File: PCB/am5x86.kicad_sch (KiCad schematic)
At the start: 2 parts, among them U1 LFE5U-25F-6BG256C, U3 AM5x86 PQFP208

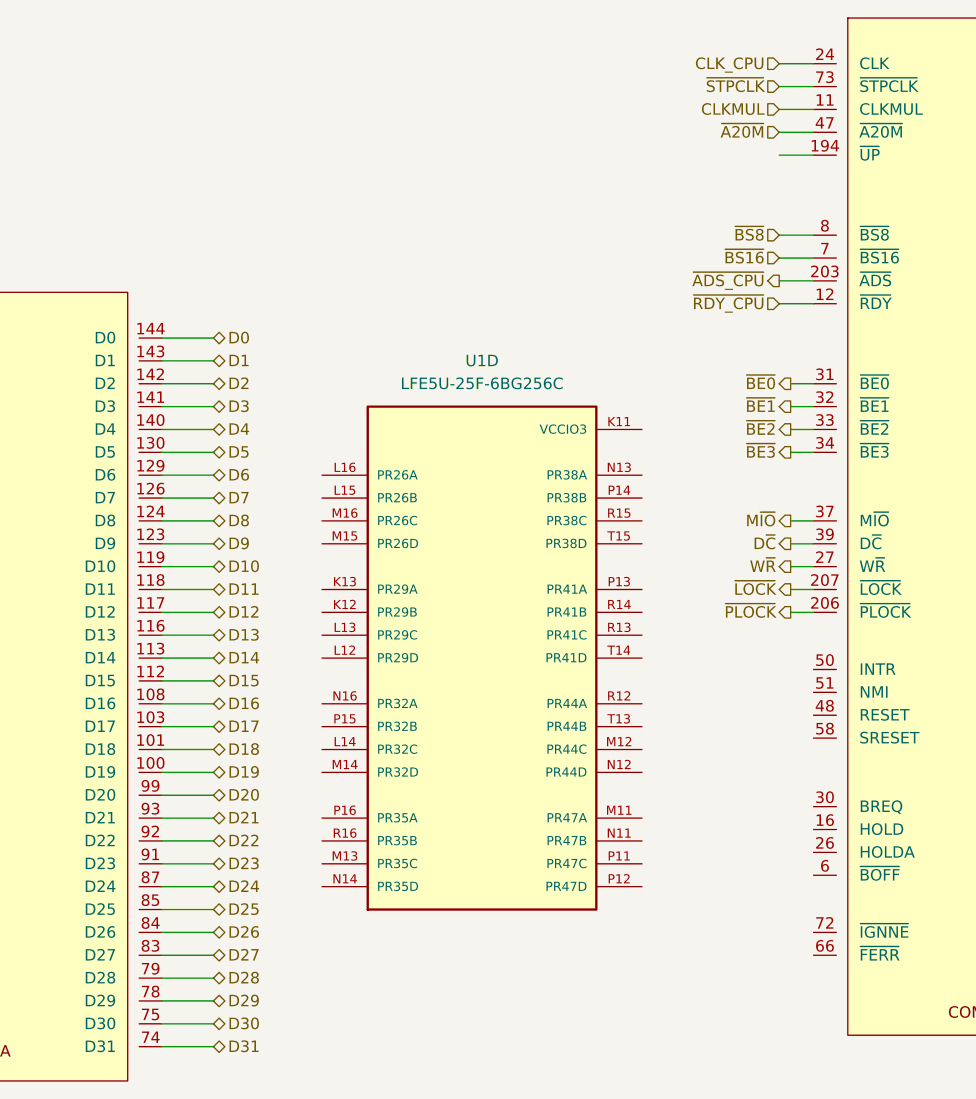
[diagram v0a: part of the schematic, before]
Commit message: More layout work
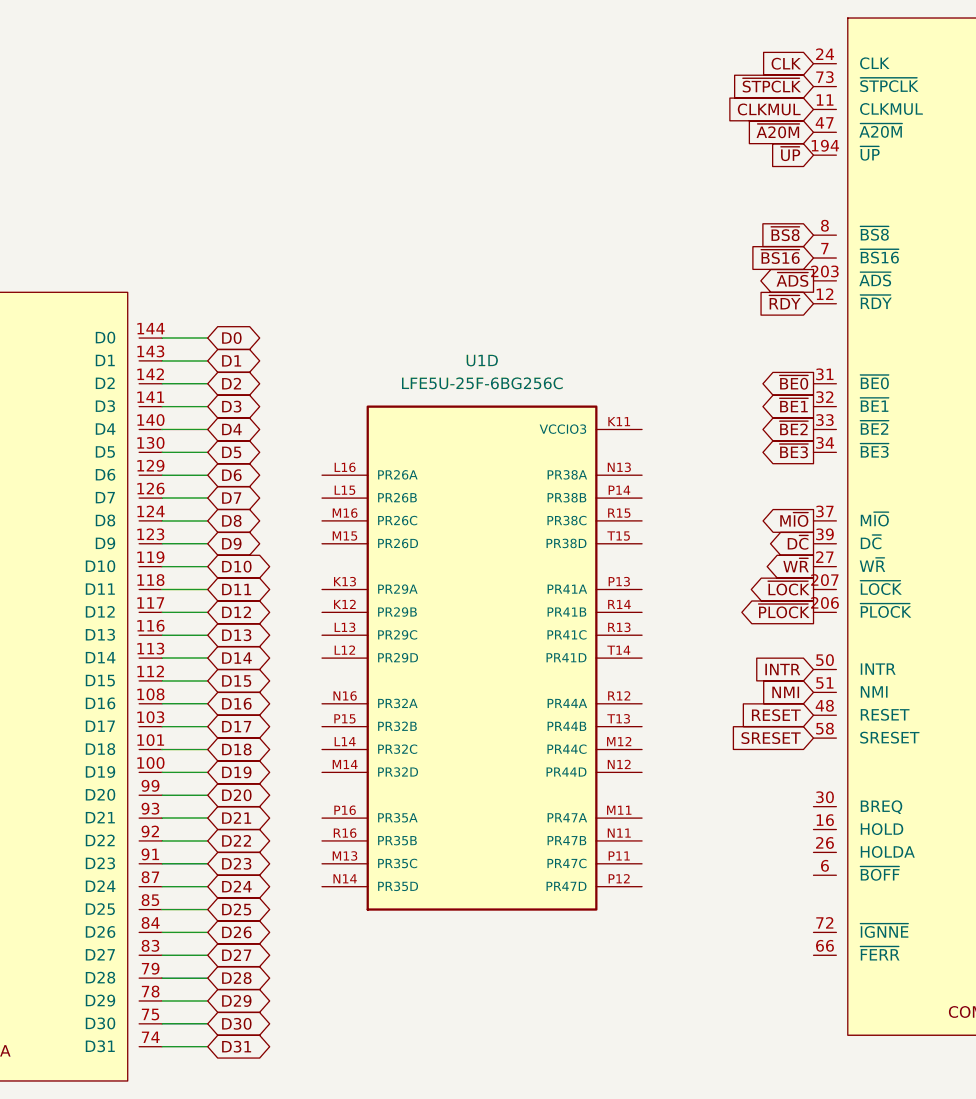
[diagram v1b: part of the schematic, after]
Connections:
- net ~{UP}: now reaches U3.194 (~{UP})
- net RESET: now reaches U3.48 (RESET)
- net INTR: now reaches U3.50 (INTR)
- net NMI: now reaches U3.51 (NMI)
- net SRESET: now reaches U3.58 (SRESET)
- net CLK_CPU renamed CLK
- net ~{ADS_CPU} renamed ~{ADS}
- net ~{RDY_CPU} renamed ~{RDY}

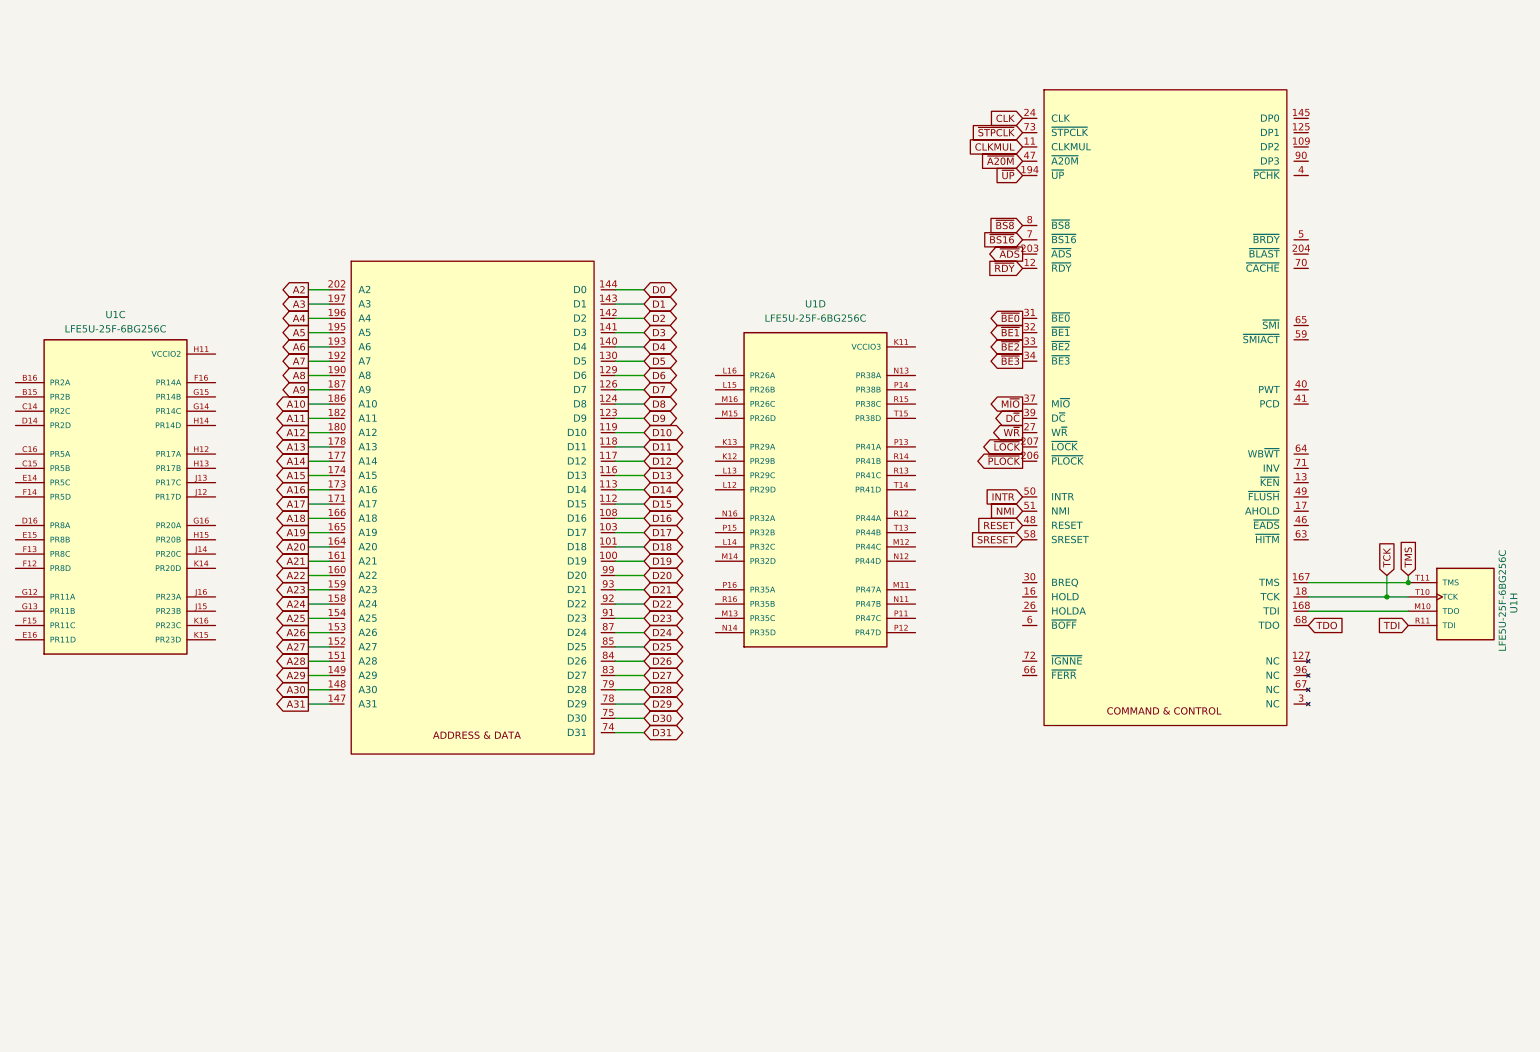
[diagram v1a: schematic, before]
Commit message: route-out in progress
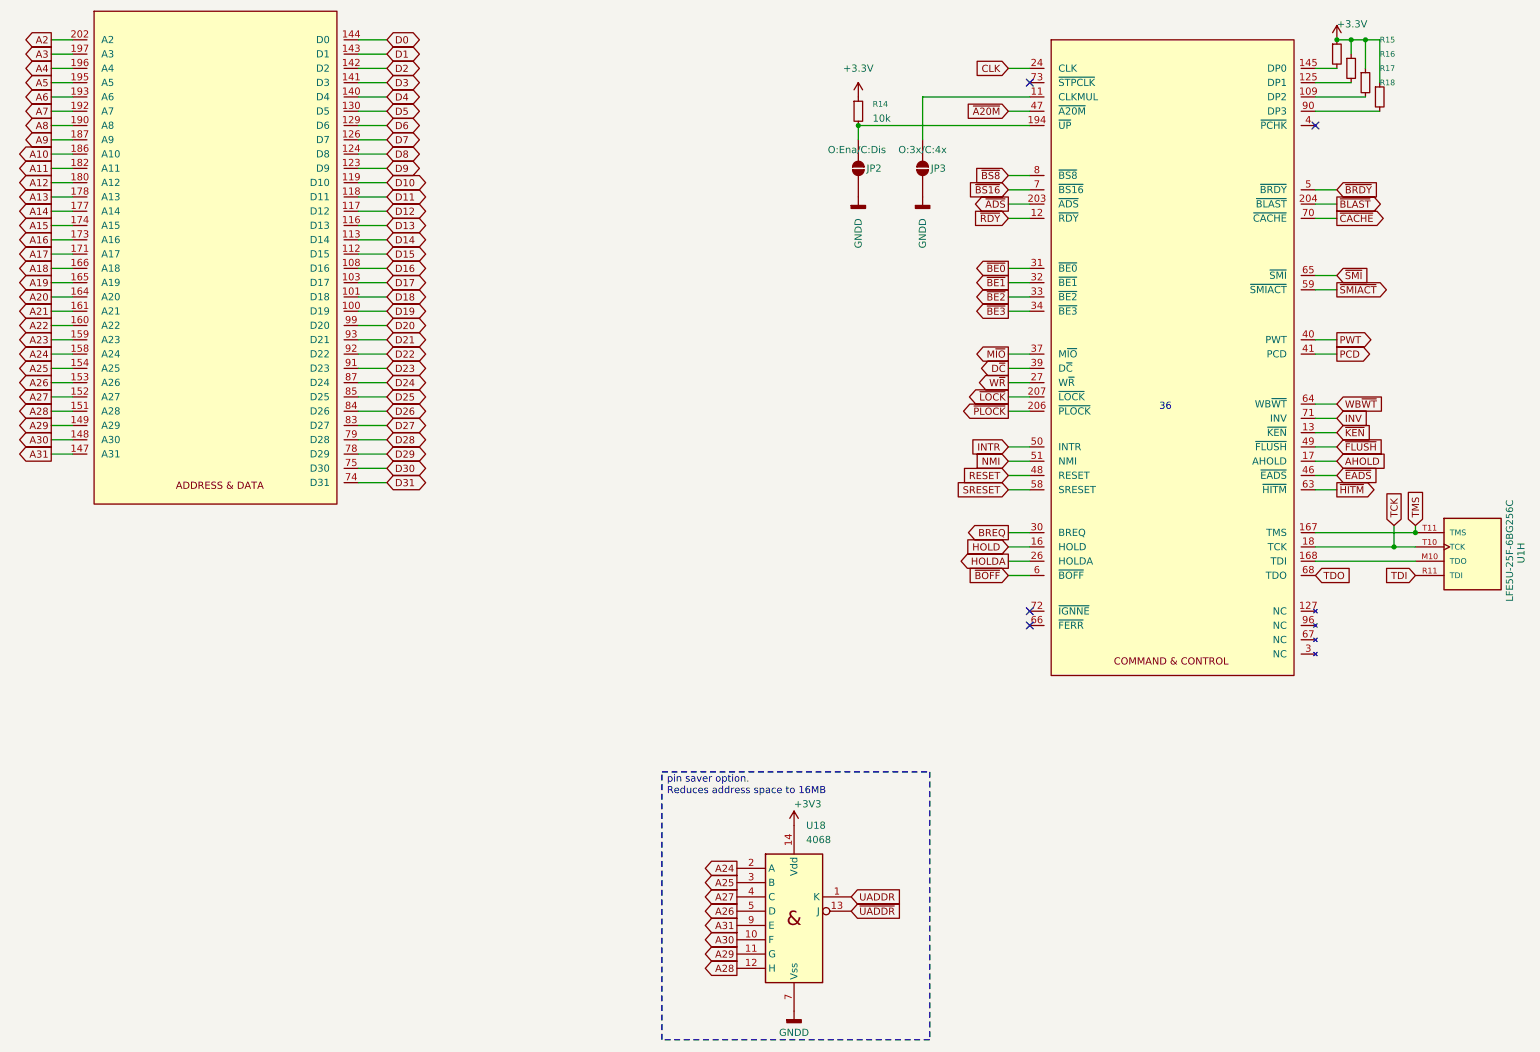
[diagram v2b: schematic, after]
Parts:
- removed unit 3 of U1
- removed unit 4 of U1
- added JP2: O:Ena/C:Dis, symbol Jumper:SolderJumper_2_Open
- added JP3: O:3x/C:4x, symbol Jumper:SolderJumper_2_Open
- added R14, R15, R16, R17, R18: 10k, symbol Device:R_Small
- added U18: 4068, Package_SO:TSSOP-14_4.4x5mm_P0.65mm, symbol 4xxx_IEEE:4068
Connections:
- net A24: now also U18.2 (A)
- net A25: now also U18.3 (B)
- net A26: now also U18.5 (D)
- net A27: now also U18.4 (C)
- net A28: now also U18.12 (H)
- net A29: now also U18.11 (G)
- net A30: now also U18.10 (F)
- net A31: now also U18.9 (E)
- net at U3.109 (DP2): now also R17.2
- net at U3.125 (DP1): now also R16.2
- net ~{KEN}: now reaches U3.13 (~{KEN})
- net at U3.145 (DP0): now also R15.2
- net HOLD: now reaches U3.16 (HOLD)
- net AHOLD: now reaches U3.17 (AHOLD)
- net ~{BLAST}: now reaches U3.204 (~{BLAST})
- net HOLDA: now reaches U3.26 (HOLDA)
- net BREQ: now reaches U3.30 (BREQ)
- net PWT: now reaches U3.40 (PWT)
- net PCD: now reaches U3.41 (PCD)
- net ~{EADS}: now reaches U3.46 (~{EADS})
- net ~{FLUSH}: now reaches U3.49 (~{FLUSH})
- net ~{BRDY}: now reaches U3.5 (~{BRDY})
- net ~{SMIACT}: now reaches U3.59 (~{SMIACT})
- net ~{BOFF}: now reaches U3.6 (~{BOFF})
- net ~{HITM}: now reaches U3.63 (~{HITM})
- net WB~{WT}: now reaches U3.64 (WB~{WT})
- net ~{SMI}: now reaches U3.65 (~{SMI})
- net ~{CACHE}: now reaches U3.70 (~{CACHE})
- net INV: now reaches U3.71 (INV)
- net at U3.90 (DP3): now also R18.2
- net CLKMUL: no longer names the net of U3.11 (CLKMUL)
- net CLKMUL: now also JP3.2 (B)
- net ~{STPCLK}: no longer names the net of U3.73 (~{STPCLK})
- net ~{UP}: no longer names the net of U3.194 (~{UP})
- net ~{UP}: now also JP2.2 (B), R14.2
- new net +3.3V: R14.1, R15.1, R16.1, R17.1, R18.1
- new net +3V3: U18.14 (Vdd)
- new net GNDD: JP2.1 (A), JP3.1 (A), U18.7 (Vss)
- new net UADDR: U18.1 (K)
- new net ~{UADDR}: U18.13 (J)
- no-connect marks 0 -> 4
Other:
- note added: "36"
- note added: "pin saver option. Reduces address space to 16MB"
- moved on the sheet: U1H
